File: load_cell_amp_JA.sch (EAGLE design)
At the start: 11 parts, among them IC2 INA122P, J1 LOAD_CELL, J2 G29

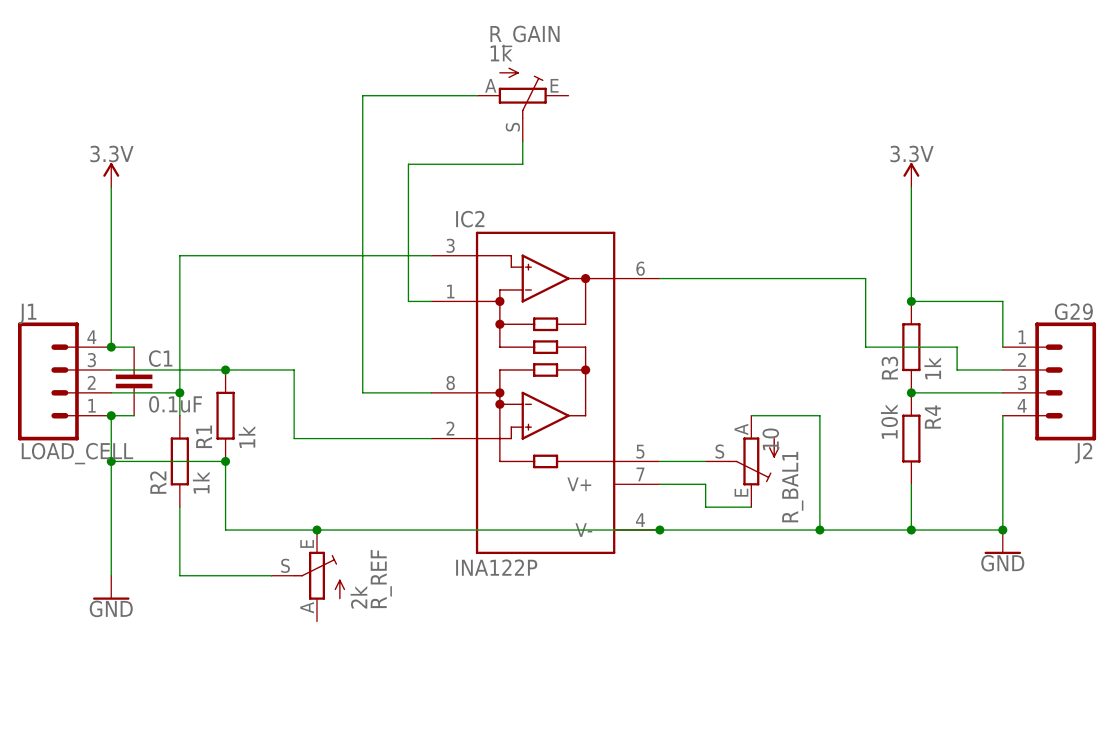
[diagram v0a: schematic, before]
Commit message: Add files via upload
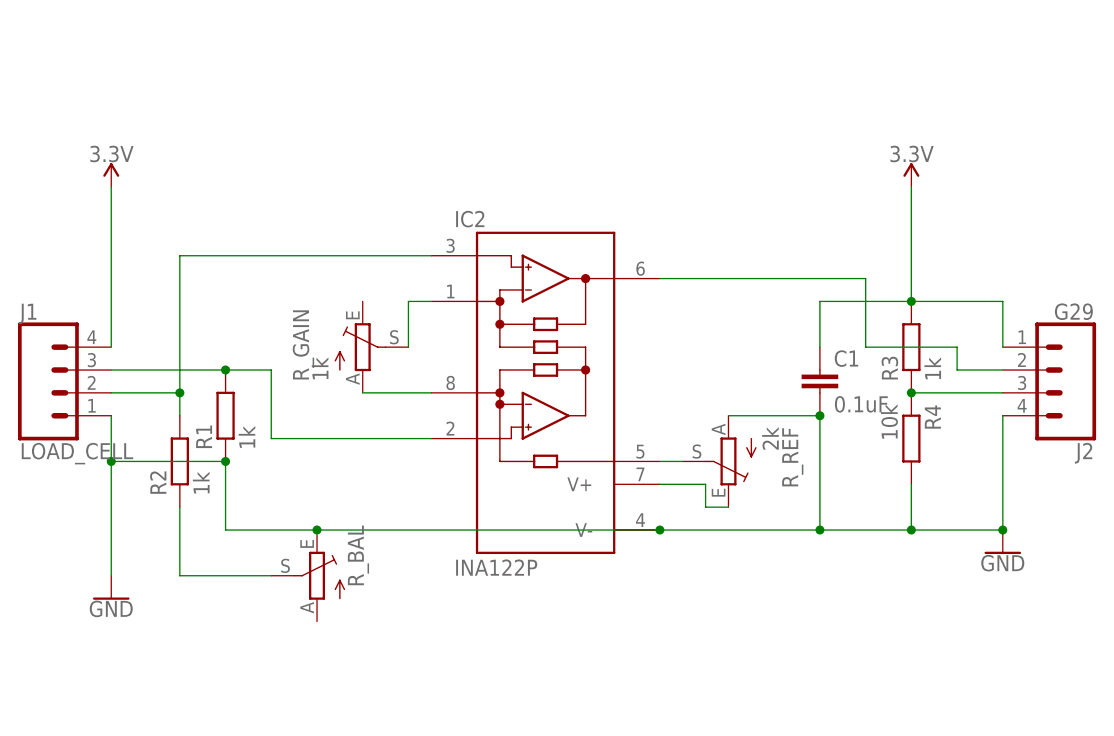
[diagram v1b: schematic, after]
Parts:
- removed R_BAL1: 10, pot:TRIM_EU-RJ9W
- added R_BAL: 10, pot:TRIM_EU-RJ9W
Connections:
- net GND: now also R_BAL.E, R_REF.A; no longer R_BAL1.A, R_REF.E
- net N$3: now also R_BAL.S; no longer R_REF.S
- net N$8: now also R_REF.E; no longer R_BAL1.E
- net N$9: now also R_REF.S; no longer R_BAL1.S
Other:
- moved on the sheet: C1, R_GAIN, R_REF

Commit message: Add files via upload
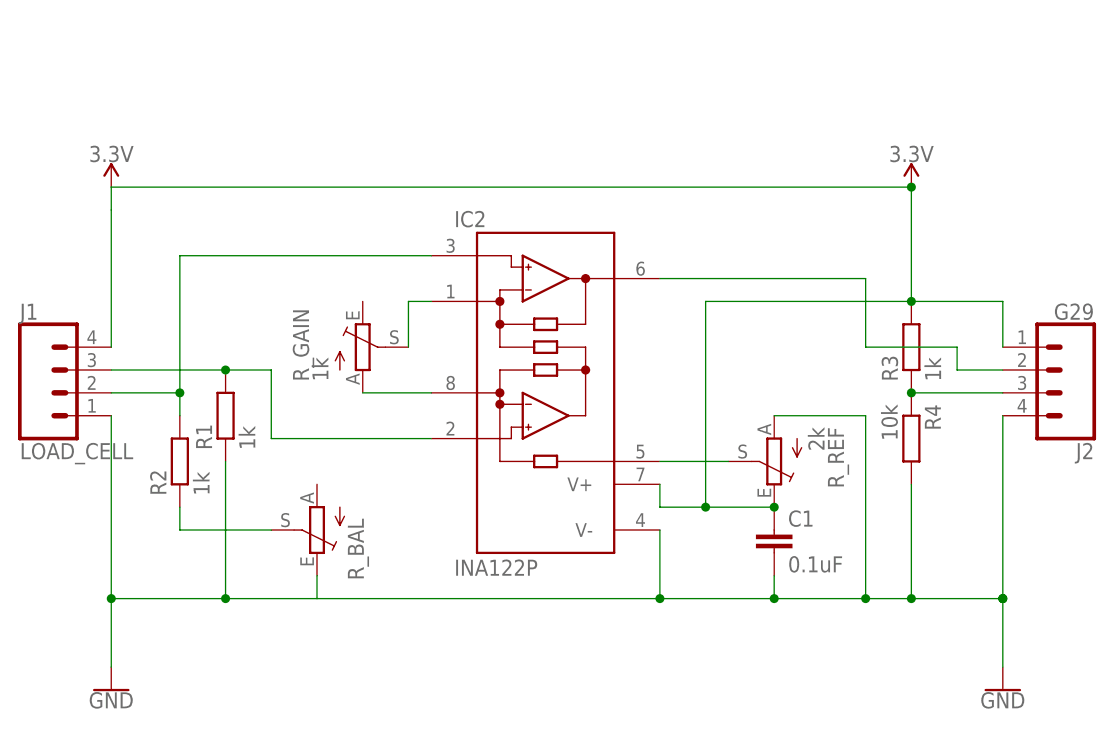
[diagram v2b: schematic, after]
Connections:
- removed net N$8: IC2.V+, R_REF.E
- net 3.3V: now also IC2.V+, R_REF.E
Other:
- moved on the sheet: C1, R_BAL, R_REF
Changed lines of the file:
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@@
 <attribute name="VALUE" x="102.362" y="62.23" size="1.778" layer="96" rot="R90"/>
 </instance>
-<instance part="C1" gate="G$1" x="88.9" y="63.5" smashed="yes">
-<attribute name="NAME" x="90.424" y="63.881" size="1.778" layer="95"/>
-<attribute name="VALUE" x="90.424" y="58.801" size="1.778" layer="96"/>
+<instance part="C1" gate="G$1" x="83.82" y="45.72" smashed="yes">
+<attribute name="NAME" x="85.344" y="46.101" size="1.778" layer="95"/>
+<attribute name="VALUE" x="85.344" y="41.021" size="1.778" layer="96"/>
 </instance>
-<instance part="GND1" gate="1" x="10.16" y="38.1" smashed="yes">
-<attribute name="VALUE" x="10.16" y="37.846" size="1.778" layer="96" align="top-center"/>
+<instance part="GND1" gate="1" x="10.16" y="27.94" smashed="yes">
+<attribute name="VALUE" x="10.16" y="27.686" size="1.778" layer="96" align="top-center"/>
 </instance>
 <instance part="SUPPLY1" gate="G$1" x="10.16" y="83.82" smashed="yes">
 <attribute name="VALUE" x="10.16" y="86.614" size="1.778" layer="96" align="bottom-center"/>
 </instance>
-<instance part="GND2" gate="1" x="109.22" y="43.18" smashed="yes">
-<attribute name="VALUE" x="109.22" y="42.926" size="1.778" layer="96" align="top-center"/>
+<instance part="GND2" gate="1" x="109.22" y="27.94" smashed="yes">
+<attribute name="VALUE" x="109.22" y="27.686" size="1.778" layer="96" align="top-center"/>
 </instance>
 <instance part="SUPPLY2" gate="G$1" x="99.06" y="83.82" smashed="yes">
 <attribute name="VALUE" x="99.06" y="86.614" size="1.778" layer="96" align="bottom-center"/>
 </instance>
-<instance part="R_BAL" gate="1" x="33.02" y="40.64" smashed="yes" rot="MR0">
-<attribute name="NAME" x="36.449" y="39.37" size="1.778" layer="95" rot="MR90"/>
+<instance part="R_BAL" gate="1" x="33.02" y="45.72" smashed="yes" rot="R180">
+<attribute name="NAME" x="36.449" y="46.99" size="1.778" layer="95" rot="R270"/>
 </instance>
-<instance part="R_REF" gate="1" x="78.74" y="53.34" smashed="yes" rot="R180">
-<attribute name="NAME" x="84.709" y="57.15" size="1.778" layer="95" rot="R270"/>
-<attribute name="VALUE" x="82.55" y="57.15" size="1.778" layer="96" rot="R270"/>
+<instance part="R_REF" gate="1" x="83.82" y="53.34" smashed="yes" rot="R180">
+<attribute name="NAME" x="89.789" y="57.15" size="1.778" layer="95" rot="R270"/>
+<attribute name="VALUE" x="87.63" y="57.15" size="1.778" layer="96" rot="R270"/>
 </instance>
 </instances>
@@
 <segment>
 <pinref part="GND1" gate="1" pin="GND"/>
+<pinref part="J1" gate="G$1" pin="1"/>
+<wire x1="10.16" y1="58.42" x2="10.16" y2="38.1" width="0.1524" layer="91"/>
 <pinref part="R1" gate="G$1" pin="1"/>
-<wire x1="22.86" y1="53.34" x2="22.86" y2="45.72" width="0.1524" layer="91"/>
-<junction x="22.86" y="53.34"/>
-<pinref part="J1" gate="G$1" pin="1"/>
-<wire x1="10.16" y1="58.42" x2="10.16" y2="53.34" width="0.1524" layer="91"/>
-<wire x1="10.16" y1="53.34" x2="22.86" y2="53.34" width="0.1524" layer="91"/>
-<junction x="10.16" y="53.34"/>
-<wire x1="10.16" y1="53.34" x2="10.16" y2="40.64" width="0.1524" layer="91"/>
+<wire x1="22.86" y1="53.34" x2="22.86" y2="38.1" width="0.1524" layer="91"/>
+<wire x1="22.86" y1="38.1" x2="10.16" y2="38.1" width="0.1524" layer="91"/>
+<junction x="10.16" y="38.1"/>
+<wire x1="10.16" y1="38.1" x2="10.16" y2="30.48" width="0.1524" layer="91"/>
+<wire x1="22.86" y1="38.1" x2="33.02" y2="38.1" width="0.1524" layer="91"/>
+<junction x="22.86" y="38.1"/>
+<pinref part="R_BAL" gate="1" pin="E"/>
+<wire x1="99.06" y1="38.1" x2="93.98" y2="38.1" width="0.1524" layer="91"/>
+<wire x1="93.98" y1="38.1" x2="83.82" y2="38.1" width="0.1524" layer="91"/>
+<wire x1="83.82" y1="38.1" x2="71.12" y2="38.1" width="0.1524" layer="91"/>
+<wire x1="71.12" y1="38.1" x2="33.02" y2="38.1" width="0.1524" layer="91"/>
+<wire x1="33.02" y1="38.1" x2="33.02" y2="40.64" width="0.1524" layer="91"/>
 <pinref part="IC2" gate="G$1" pin="V-"/>
-<wire x1="71.12" y1="45.72" x2="88.9" y2="45.72" width="0.1524" layer="91"/>
+<wire x1="71.12" y1="45.72" x2="71.12" y2="38.1" width="0.1524" layer="91"/>
+<junction x="71.12" y="38.1"/>
+<pinref part="R4" gate="G$1" pin="2"/>
+<wire x1="99.06" y1="50.8" x2="99.06" y2="38.1" width="0.1524" layer="91"/>
 <pinref part="J2" gate="G$1" pin="4"/>
-<wire x1="88.9" y1="45.72" x2="99.06" y2="45.72" width="0.1524" layer="91"/>
-<wire x1="99.06" y1="45.72" x2="109.22" y2="45.72" width="0.1524" layer="91"/>
-<wire x1="109.22" y1="45.72" x2="109.22" y2="58.42" width="0.1524" layer="91"/>
-<pinref part="R4" gate="G$1" pin="2"/>
-<wire x1="99.06" y1="50.8" x2="99.06" y2="45.72" width="0.1524" layer="91"/>
-<junction x="99.06" y="45.72"/>
+<wire x1="109.22" y1="30.48" x2="109.22" y2="38.1" width="0.1524" layer="91"/>
 <pinref part="GND2" gate="1" pin="GND"/>
-<junction x="109.22" y="45.72"/>
-<wire x1="22.86" y1="45.72" x2="33.02" y2="45.72" width="0.1524" layer="91"/>
-<junction x="71.12" y="45.72"/>
-<pinref part="R_BAL" gate="1" pin="E"/>
-<wire x1="33.02" y1="45.72" x2="71.12" y2="45.72" width="0.1524" layer="91"/>
-<junction x="33.02" y="45.72"/>
+<wire x1="109.22" y1="38.1" x2="109.22" y2="58.42" width="0.1524" layer="91"/>
+<wire x1="99.06" y1="38.1" x2="109.22" y2="38.1" width="0.1524" layer="91"/>
+<junction x="99.06" y="38.1"/>
+<junction x="109.22" y="38.1"/>
 <pinref part="R_REF" gate="1" pin="A"/>
-<wire x1="78.74" y1="58.42" x2="88.9" y2="58.42" width="0.1524" layer="91"/>
-<wire x1="88.9" y1="58.42" x2="88.9" y2="45.72" width="0.1524" layer="91"/>
-<junction x="88.9" y="45.72"/>
+<wire x1="83.82" y1="58.42" x2="93.98" y2="58.42" width="0.1524" layer="91"/>
+<wire x1="93.98" y1="58.42" x2="93.98" y2="38.1" width="0.1524" layer="91"/>
+<junction x="93.98" y="38.1"/>
 <pinref part="C1" gate="G$1" pin="2"/>
-<junction x="88.9" y="58.42"/>
+<wire x1="83.82" y1="40.64" x2="83.82" y2="38.1" width="0.1524" layer="91"/>
+<junction x="83.82" y="38.1"/>
+</segment>
+<segment>
+<junction x="109.22" y="38.1"/>
 </segment>
 </net>
@@
 <net name="3.3V" class="0">
 <segment>
+<pinref part="J1" gate="G$1" pin="4"/>
+<pinref part="SUPPLY1" gate="G$1" pin="3.3V"/>
+<wire x1="10.16" y1="66.04" x2="10.16" y2="81.28" width="0.1524" layer="91"/>
 <pinref part="R3" gate="G$1" pin="2"/>
 <wire x1="99.06" y1="71.12" x2="109.22" y2="71.12" width="0.1524" layer="91"/>
@@
 <wire x1="99.06" y1="71.12" x2="99.06" y2="83.82" width="0.1524" layer="91"/>
 <junction x="99.06" y="71.12"/>
+<pinref part="IC2" gate="G$1" pin="V+"/>
+<wire x1="71.12" y1="48.26" x2="71.12" y2="50.8" width="0.1524" layer="91"/>
+<pinref part="R_REF" gate="1" pin="E"/>
+<wire x1="83.82" y1="48.26" x2="76.2" y2="48.26" width="0.1524" layer="91"/>
 <pinref part="C1" gate="G$1" pin="1"/>
-<wire x1="88.9" y1="66.04" x2="88.9" y2="71.12" width="0.1524" layer="91"/>
-<wire x1="88.9" y1="71.12" x2="99.06" y2="71.12" width="0.1524" layer="91"/>
-</segment>
-<segment>
-<pinref part="J1" gate="G$1" pin="4"/>
-<pinref part="SUPPLY1" gate="G$1" pin="3.3V"/>
-<wire x1="10.16" y1="66.04" x2="10.16" y2="83.82" width="0.1524" layer="91"/>
+<junction x="83.82" y="48.26"/>
+<wire x1="76.2" y1="48.26" x2="71.12" y2="48.26" width="0.1524" layer="91"/>
+<wire x1="76.2" y1="48.26" x2="76.2" y2="71.12" width="0.1524" layer="91"/>
+<wire x1="76.2" y1="71.12" x2="99.06" y2="71.12" width="0.1524" layer="91"/>
+<junction x="76.2" y="48.26"/>
+<wire x1="10.16" y1="81.28" x2="10.16" y2="83.82" width="0.1524" layer="91"/>
+<wire x1="10.16" y1="83.82" x2="99.06" y2="83.82" width="0.1524" layer="91"/>
+<junction x="99.06" y="83.82"/>
 </segment>
 </net>
@@
 </segment>
 </net>
-<net name="N$8" class="0">
+<net name="N$9" class="0">
 <segment>
-<wire x1="76.2" y1="48.26" x2="76.2" y2="50.8" width="0.1524" layer="91"/>
-<pinref part="IC2" gate="G$1" pin="V+"/>
-<wire x1="76.2" y1="50.8" x2="71.12" y2="50.8" width="0.1524" layer="91"/>
-<pinref part="R_REF" gate="1" pin="E"/>
-<wire x1="78.74" y1="48.26" x2="76.2" y2="48.26" width="0.1524" layer="91"/>
+<pinref part="IC2" gate="G$1" pin="REF"/>
+<pinref part="R_REF" gate="1" pin="S"/>
+<wire x1="71.12" y1="53.34" x2="78.74" y2="53.34" width="0.1524" layer="91"/>
 </segment>
 </net>
@@
 <segment>
 <pinref part="R2" gate="G$1" pin="1"/>
-<wire x1="17.78" y1="48.26" x2="17.78" y2="40.64" width="0.1524" layer="91"/>
+<wire x1="17.78" y1="48.26" x2="17.78" y2="45.72" width="0.1524" layer="91"/>
 <pinref part="R_BAL" gate="1" pin="S"/>
-<wire x1="17.78" y1="40.64" x2="27.94" y2="40.64" width="0.1524" layer="91"/>
+<wire x1="17.78" y1="45.72" x2="27.94" y2="45.72" width="0.1524" layer="91"/>
 </segment>
 </net>
-<net name="N$9" class="0">
-<segment>
-<pinref part="IC2" gate="G$1" pin="REF"/>
-<pinref part="R_REF" gate="1" pin="S"/>
-<wire x1="71.12" y1="53.34" x2="73.66" y2="53.34" width="0.1524" layer="91"/>
-</segment>
-</net>
